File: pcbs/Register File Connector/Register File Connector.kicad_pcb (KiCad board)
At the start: 2 copper layers, 4 parts, among them J101 Conn_02x20_Odd_Even, J102 Conn_02x20_Odd_Even, J103 Conn_01x04, J104 Conn_02x20_Odd_Even

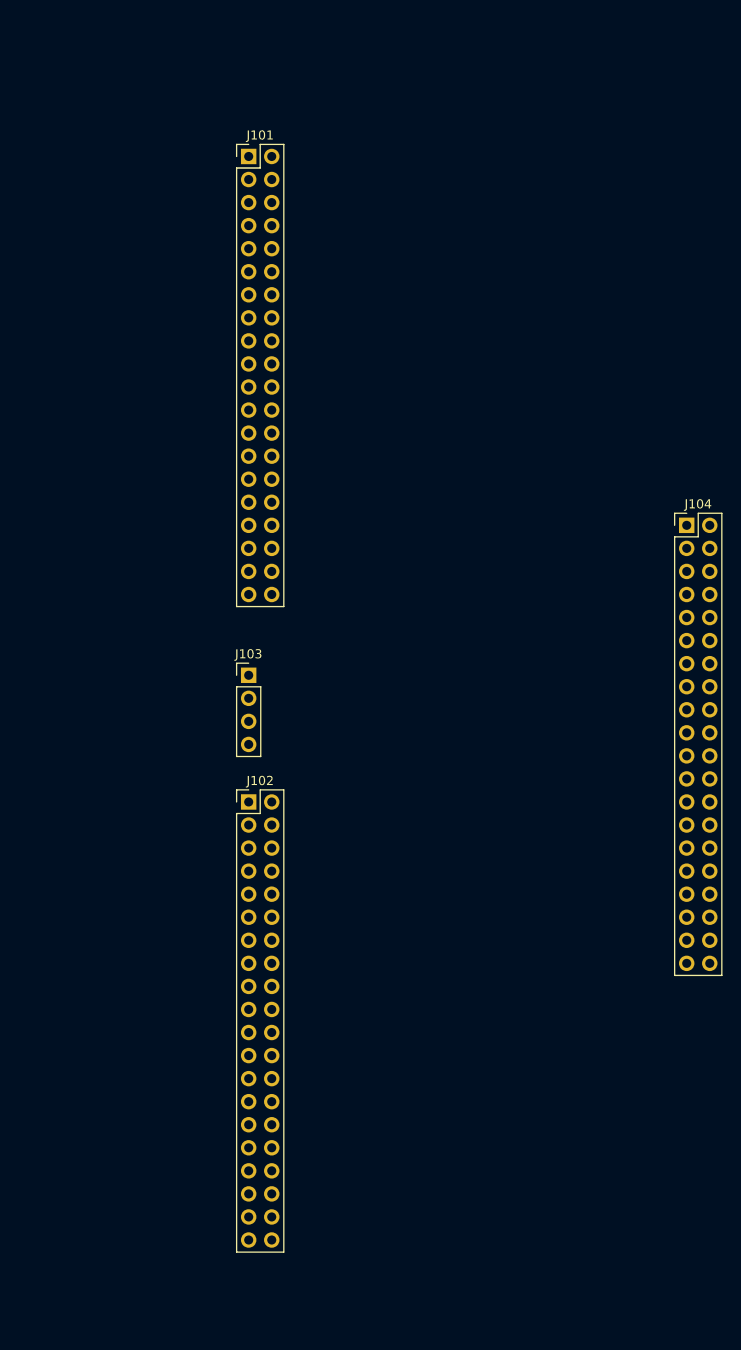
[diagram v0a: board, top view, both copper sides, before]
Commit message: Put together the connector
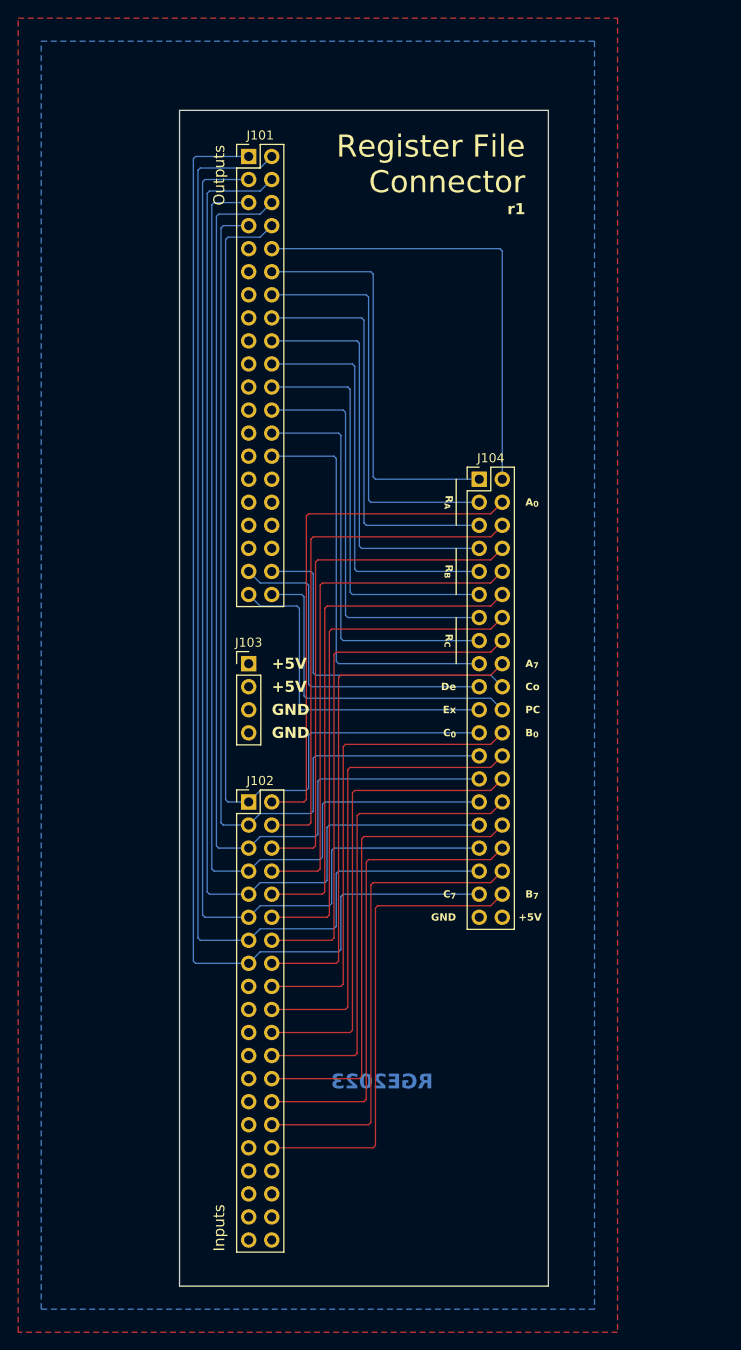
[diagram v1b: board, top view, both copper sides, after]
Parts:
- moved J104 23.4 mm to (101.6, 86.4)
- moved J103 1.28 mm to (76.2, 106.7)
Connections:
- J101 pad 1: /C_{0} -> /C_{7}
- J101 pad 10: /R_{A}0 -> /C_{W}/~{C_{R}}
- J101 pad 12: /R_{A}1 -> /R_{A}0
- J101 pad 14: /R_{A}2 -> /R_{A}1
- J101 pad 16: /R_{B}0 -> /R_{A}2
- J101 pad 18: /R_{B}1 -> /R_{B}0
- J101 pad 2: /C_{4} -> /C_{6}
- J101 pad 20: /R_{B}2 -> /R_{B}1
- J101 pad 22: /R_{C}0 -> /R_{B}2
- J101 pad 24: /R_{C}1 -> /R_{C}0
- J101 pad 26: /R_{C}2 -> /R_{C}1
- J101 pad 28: unconnected-(J101-Pin_28-Pad28) -> /R_{C}2
- J101 pad 3: /C_{1} -> /C_{5}
- J101 pad 33: /Decode -> unconnected-(J101-Pin_33-Pad33)
- J101 pad 35: /Execute -> unconnected-(J101-Pin_35-Pad35)
- J101 pad 37: /Commit -> /Decode
- J101 pad 38: unconnected-(J101-Pin_38-Pad38) -> /Commit
- J101 pad 39: /PC Update -> /Execute
- J101 pad 4: /C_{5} -> /C_{4}
- J101 pad 40: /C_{W}/~{C_{R}} -> /PC Update
- J101 pad 5: /C_{2} -> /C_{3}
- J101 pad 6: /C_{6} -> /C_{2}
- J101 pad 7: /C_{3} -> /C_{1}
- J101 pad 8: /C_{7} -> /C_{0}
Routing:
- net /C_{7}: track 0.00 -> 132.8 mm
- net /C_{6}: track 0.00 -> 131.0 mm
- net /C_{5}: track 0.00 -> 123.1 mm
- net /C_{4}: track 0.00 -> 121.4 mm
- net /C_{3}: track 0.00 -> 113.5 mm
- net /C_{2}: track 0.00 -> 111.7 mm
- net /C_{1}: track 0.00 -> 103.8 mm
- net /C_{0}: track 0.00 -> 102.1 mm
- net /A_{5}: track 0.00 -> 57.4 mm
- net /A_{4}: track 0.00 -> 57.4 mm
- net /A_{1}: track 0.00 -> 57.4 mm
- net /A_{6}: track 0.00 -> 57.4 mm
- net /A_{3}: track 0.00 -> 57.4 mm
- net /A_{2}: track 0.00 -> 57.4 mm
- net /A_{0}: track 0.00 -> 57.4 mm
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- added copper zone on B.Cu, net +5V
- added copper zone on F.Cu, net GND
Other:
- board outline added: 40.6 x 129.5 mm
- board text added: "+5V"
- board text added: "A_{0}"
- board text added: "A_{7}"
- board text added: "B_{0}"
- board text added: "B_{7}"
- board text added: "C_{0}"
- board text added: "C_{7}"
- board text added: "Co"
- board text added: "De"
- board text added: "Ex"
- board text added: "GND"
- board text added: "Inputs"
- board text added: "JLCJLCJLCJLC"
- board text added: "Outputs"
- board text added: "PC"
- board text added: "RGE2023"
- board text added: "R_{A}"
- board text added: "R_{B}"
- board text added: "R_{C}"
- board text added: "Register File Connector"
- board text added: "r${REVISION}"
